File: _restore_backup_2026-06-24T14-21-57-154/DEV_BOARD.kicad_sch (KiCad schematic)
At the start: 34 parts, among them J1 USB_C_Receptacle_USB2.0_16P, J2 Conn_ARM_SWD_TagConnect_TC2030, U1 MSPM0G350x, U2 USBLC6-2SC6, U3 SPX3819M5-L-3-3, U4 CH340E, U5 LIS2DH, X1 8MHz

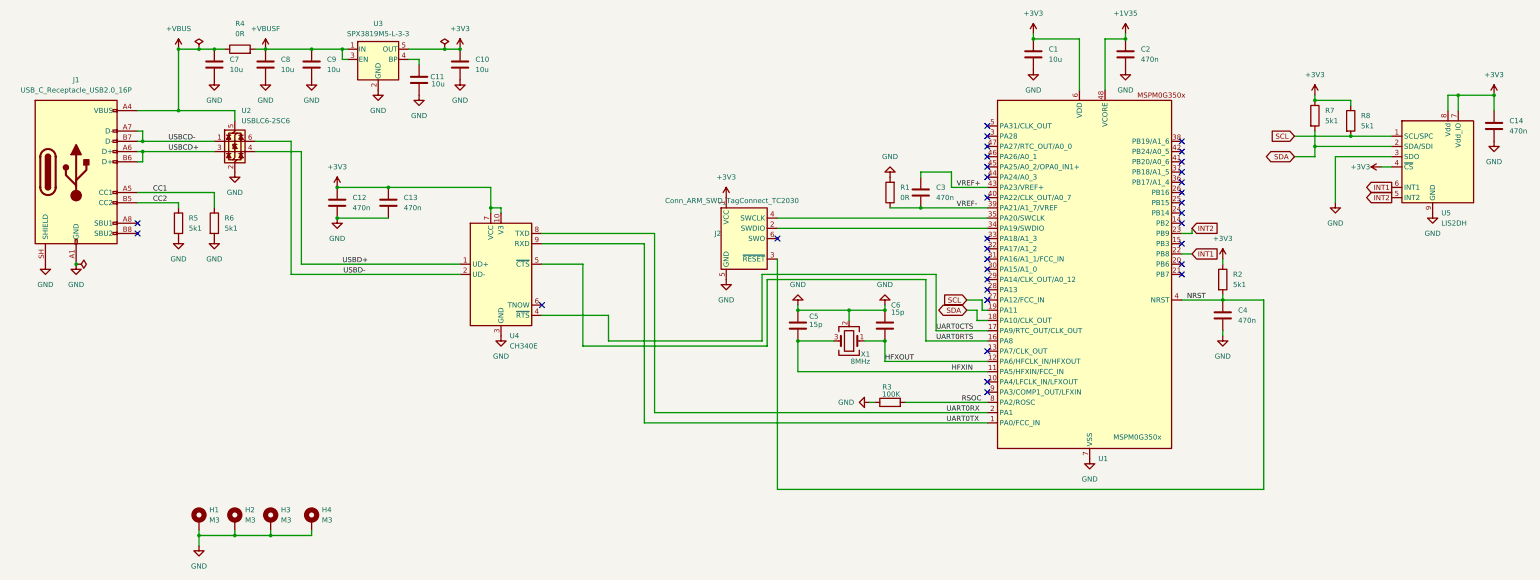
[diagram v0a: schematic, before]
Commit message: Routing completed
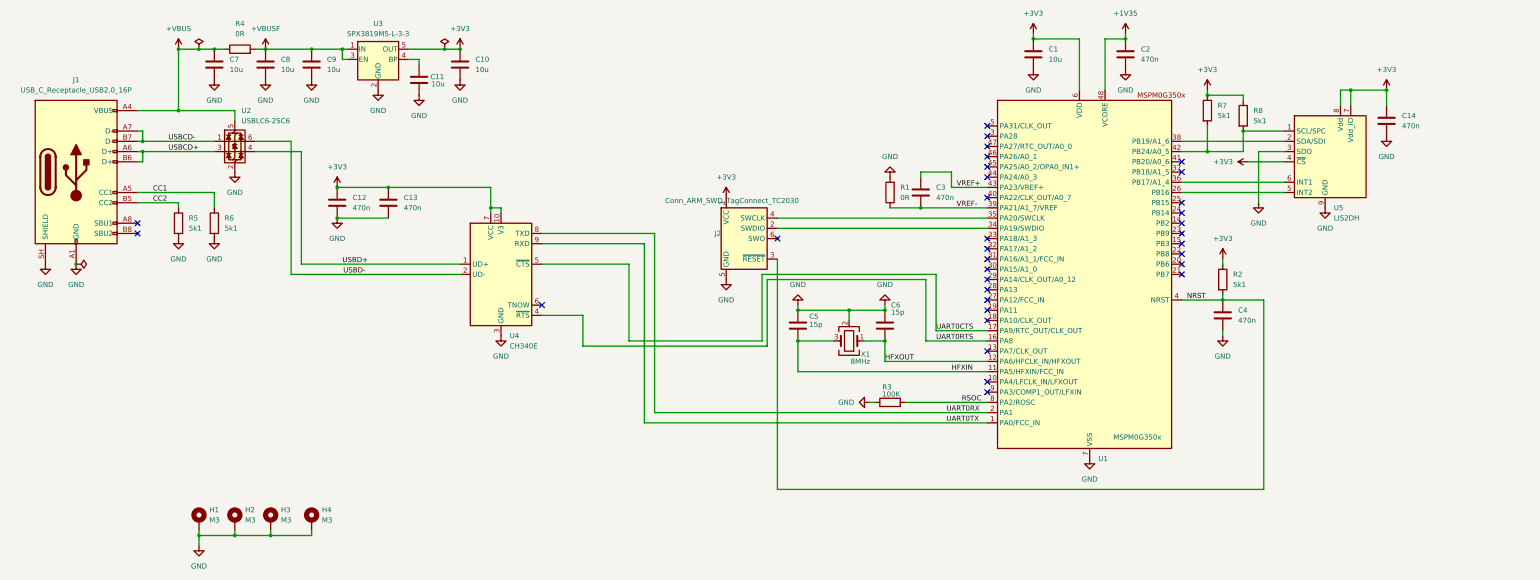
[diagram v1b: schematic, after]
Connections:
- net UART0CTS: now also U4.5 (~{CTS}); no longer U4.4 (~{RTS})
- net UART0RTS: now also U4.4 (~{RTS}); no longer U4.5 (~{CTS})
- net at U1.26 (PB16): now also U5.5 (INT2)
- net at U1.36 (PB17/A1_4): now also U5.6 (INT1)
- net at U1.38 (PB19/A1_6): now also U5.2 (SDA/SDI)
- net at U1.42 (PB24/A0_5): now also R7.2, R8.2, U5.1 (SCL/SPC)
- net INT1: no longer names the net of U1.22 (PB8)
- net INT1: no longer U5.6 (INT1)
- net INT2: no longer names the net of U1.23 (PB9)
- net INT2: no longer U5.5 (INT2)
- removed net SCL: R8.2, U1.19 (PA11), U5.1 (SCL/SPC)
- removed net SDA: R7.2, U1.18 (PA10/CLK_OUT), U5.2 (SDA/SDI)
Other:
- moved on the sheet: C14, R7, R8, U5
